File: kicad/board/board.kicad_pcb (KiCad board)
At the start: 2 copper layers, 126.9 x 103.7 mm, 44 parts

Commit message: we messed up pcb
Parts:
- added S20: SSSS811101, sCLACKEN:SW_SSSS811101, B.Cu at (255.0, 154.5)
- D1, D10, D11, D12, D13, D14, D15, D16, D17, D18, D2, D3, D4, D5, D6, D7, D8, D9: value 1N914 -> D
- H1, H2, H3, H4: value MountingHole_2.2mm_M2 -> MountingHole
- S1, S10, S11, S12, S13, S14, S15, S16, S17, S18, S2, S3, S4, S5, S6, S7, S8, S9: value SW_Push_45deg -> SW_SPST
- S19: value SW_SSSS811101 -> SSSS811101
- U1: value (none) -> ~; footprint xiao-ble-tht -> clacken:seeed_xaio
- moved S19 228.4 mm to (255.0, 154.5)
- moved D11 220.4 mm to (216.0, 141.2)
- moved D12 220.4 mm to (217.6, 123.3)
- moved D14 220.4 mm to (233.8, 144.8)
- moved D15 220.4 mm to (235.3, 126.9)
- moved D18 220.4 mm to (258.2, 197.0)
- moved D3 220.4 mm to (159.4, 127.3)
- moved D7 220.4 mm to (197.1, 150.6)
- moved D9 220.4 mm to (200.2, 114.8)
- moved H2 220.4 mm to (228.3, 127.6)
- moved H3 220.4 mm to (152.5, 128.6)
- moved H4 220.4 mm to (152.5, 164.6)
- moved JST1 220.4 mm to (239.6, 141.1)
- moved JST2 220.4 mm to (254.6, 142.4)
- moved S1 220.4 mm to (152.5, 159.1)
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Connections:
- D1 pad 1: Row3 -> G2
- D10 pad 1: Row3 -> G2
- D11 pad 1: Row2 -> G1
- D12 pad 1: Row1 -> G0
- D13 pad 1: Row3 -> G2
- D14 pad 1: Row2 -> G1
- D15 pad 1: Row1 -> G0
- D16 pad 1: Row4 -> G3
- D17 pad 1: Row4 -> G3
- D18 pad 1: Row4 -> G3
- D2 pad 1: Row2 -> G1
- D3 pad 1: Row1 -> G0
- D4 pad 1: Row3 -> G2
- D5 pad 1: Row2 -> G1
- D6 pad 1: Row1 -> G0
- D7 pad 1: Row3 -> G2
- D8 pad 1: Row2 -> G1
- D9 pad 1: Row1 -> G0
- JST2 pad 1: Net-(JST1-Pin_1) -> Net-(JST1-Pin_2)
- JST2 pad 2: Net-(JST1-Pin_2) -> Net-(JST2-Pin_2)
- S1 pad 1: Col1 -> Net-(D1-A)
- S1 pad 2: Net-(D1-A) -> C0
- S10 pad 1: Col4 -> Net-(D10-A)
- S10 pad 2: Net-(D10-A) -> C3
- S11 pad 1: Col4 -> Net-(D11-A)
- S11 pad 2: Net-(D11-A) -> C3
- S12 pad 1: Col4 -> Net-(D12-A)
- S12 pad 2: Net-(D12-A) -> C3
- S13 pad 1: Col5 -> Net-(D13-A)
- S13 pad 2: Net-(D13-A) -> C4
- S14 pad 1: Col5 -> Net-(D14-A)
- S14 pad 2: Net-(D14-A) -> C4
- S15 pad 1: Col5 -> Net-(D15-A)
- S15 pad 2: Net-(D15-A) -> C4
- S16 pad 1: Col3 -> Net-(D16-A)
- S16 pad 2: Net-(D16-A) -> C2
- S17 pad 1: Col4 -> Net-(D17-A)
- S17 pad 2: Net-(D17-A) -> C3
- S18 pad 1: Col5 -> Net-(D18-A)
- S18 pad 2: Net-(D18-A) -> C4
- S19 pad 1: (no net) -> unconnected-(S19-Pad1)
- S19 pad 2: (no net) -> Net-(JST1-Pin_1)
- S19 pad 3: (no net) -> Net-(JST2-Pin_2)
- S2 pad 1: Col1 -> Net-(D2-A)
- S2 pad 2: Net-(D2-A) -> C0
- S3 pad 1: Col1 -> Net-(D3-A)
- S3 pad 2: Net-(D3-A) -> C0
- S4 pad 1: Col2 -> Net-(D4-A)
- S4 pad 2: Net-(D4-A) -> C1
- S5 pad 1: Col2 -> Net-(D5-A)
- S5 pad 2: Net-(D5-A) -> C1
- S6 pad 1: Col2 -> Net-(D6-A)
- S6 pad 2: Net-(D6-A) -> C1
- S7 pad 1: Col3 -> Net-(D7-A)
- S7 pad 2: Net-(D7-A) -> C2
- S8 pad 1: Col3 -> Net-(D8-A)
- S8 pad 2: Net-(D8-A) -> C2
- S9 pad 1: Col3 -> Net-(D9-A)
- S9 pad 2: Net-(D9-A) -> C2
- U1 pad 0: P0 -> unconnected-(U1-P0-Pad0)_2
- U1 pad 1: P1 -> unconnected-(U1-P1-Pad1)_2
- U1 pad 10: P10 -> G0
- U1 pad 11: _1_11 -> unconnected-(U1-V3-Pad11)_1
- U1 pad 12: _1_12 -> unconnected-(U1-GND-Pad12)_1
- U1 pad 13: _1_13 -> unconnected-(U1-VCC-Pad13)
- U1 pad 2: P2 -> C0
- U1 pad 3: P3 -> C1
- U1 pad 4: P4 -> C2
- U1 pad 5: P5 -> C3
- U1 pad 6: P6 -> C4
- U1 pad 7: P7 -> G3
- U1 pad 8: P8 -> G2
- U1 pad 9: P9 -> G1
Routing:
- net C0: track 0.00 -> 214.5 mm, vias 0 -> 3
- net C2: track 0.00 -> 201.0 mm, vias 0 -> 4
- net C3: track 0.00 -> 186.1 mm, vias 0 -> 7
- net C1: track 0.00 -> 165.6 mm, vias 0 -> 3
- net C4: track 0.00 -> 155.1 mm, vias 0 -> 6
- net G3: track 0.00 -> 123.5 mm
- net G0: track 0.00 -> 122.3 mm
- net G1: track 0.00 -> 120.6 mm
- net G2: track 0.00 -> 100.1 mm
- net (no net): track 0.00 -> 99.6 mm
- net Net-(JST1-Pin_1): track 0.00 -> 28.5 mm, vias 0 -> 1
- net Net-(JST1-Pin_2): track 0.00 -> 15.5 mm
- net Net-(JST2-Pin_2): track 0.00 -> 10.3 mm
- net VCC: track 10.3 -> 0.00 mm
- net P0: track 10.3 -> 0.00 mm
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
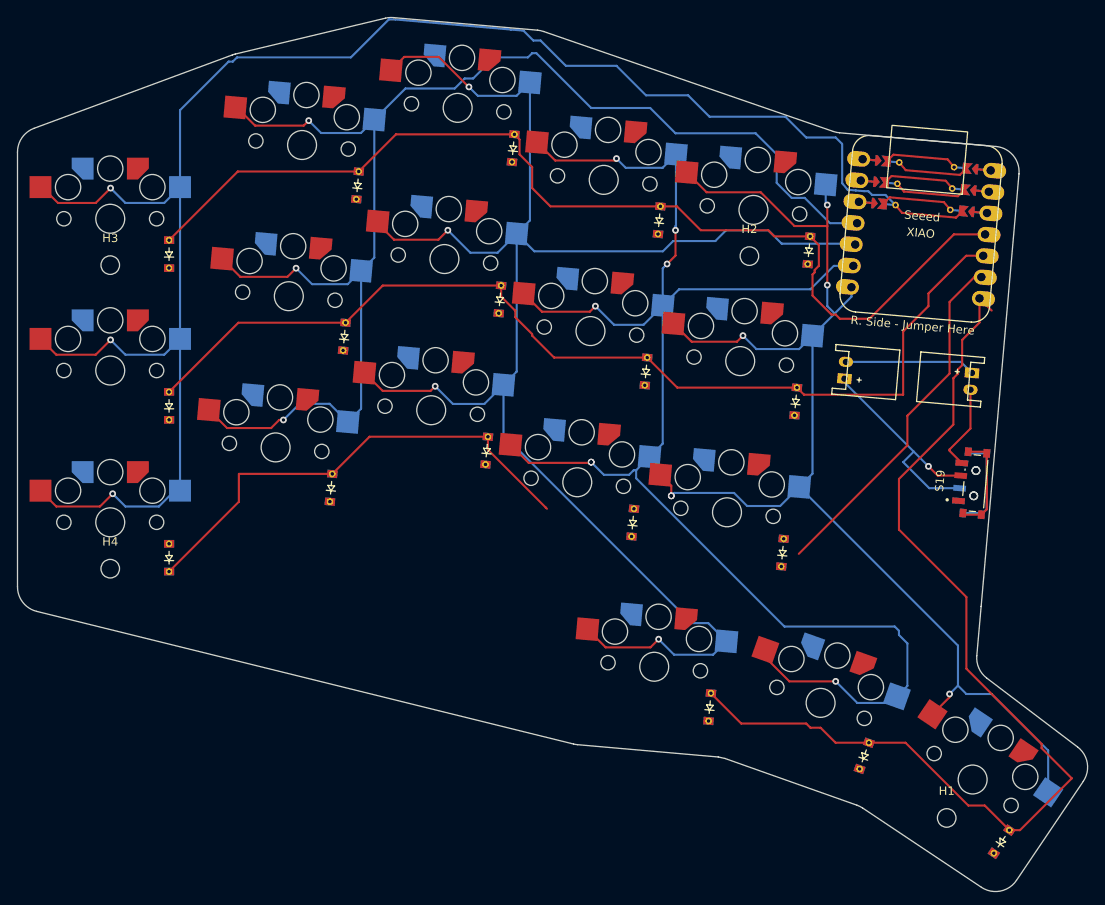
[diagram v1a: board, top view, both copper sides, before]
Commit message: traces
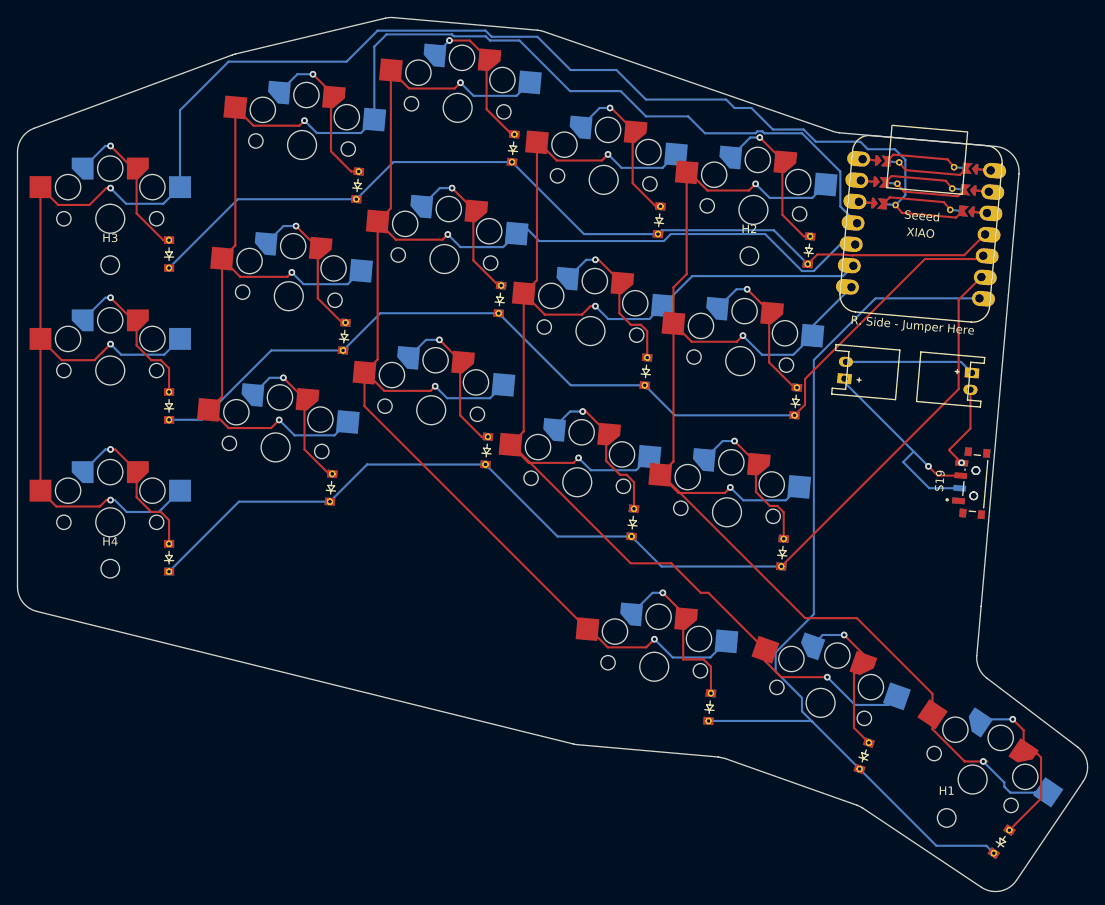
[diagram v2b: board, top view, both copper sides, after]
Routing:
- net G2: track 100.1 -> 127.0 mm
- net (no net): track 99.6 -> 75.5 mm
- net Net-(D18-A): track 0.00 -> 21.3 mm, vias 0 -> 1
- net Net-(D16-A): track 0.00 -> 20.8 mm, vias 0 -> 1
- net Net-(D11-A): track 0.00 -> 19.6 mm, vias 0 -> 1
- net Net-(D2-A): track 0.00 -> 19.6 mm, vias 0 -> 1
- net Net-(D1-A): track 0.00 -> 19.6 mm, vias 0 -> 1
- net Net-(D10-A): track 0.00 -> 19.6 mm, vias 0 -> 1
- net Net-(D6-A): track 0.00 -> 19.5 mm, vias 0 -> 1
- net Net-(D15-A): track 0.00 -> 19.5 mm, vias 0 -> 1
- net Net-(D13-A): track 0.00 -> 19.4 mm, vias 0 -> 1
- net Net-(D17-A): track 0.00 -> 19.4 mm, vias 0 -> 1
- net Net-(D12-A): track 0.00 -> 19.3 mm, vias 0 -> 1
- net Net-(D3-A): track 0.00 -> 19.3 mm, vias 0 -> 1
- net Net-(D7-A): track 0.00 -> 19.3 mm, vias 0 -> 1
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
